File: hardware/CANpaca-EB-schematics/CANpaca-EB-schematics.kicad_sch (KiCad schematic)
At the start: 132 parts, among them J11 Conn_01x03_Male, J12 A2501WV-4P, J13 A2501WV-3P, J14 A2501WV-5P, J16 A2501WV-3P, J17 A2501WV-2P, J2 FAN_0, J4 Conn_01x03_Male, J5 FAN_1, J6 Screw_Terminal_01x02, J7 Conn_02x02_Odd_Even, J8 A2501WV-4P, J9 USB4110-GF-A_REVB, Q1 ES34000, Q2 ES34000, Q3 PSMN5R2-60YL, SW1 SW_DIP_x08, U1 SN65HVD1050D, U10 RP2040, U11 ADXL343, U2 SN74LVC1G14DRL, U3 TMC2130-LA, U4 LN5016, U5 AMS1117-3.3, U6 W25Q16, U7 USBLC6-2SC6, U8 MAX31865xTP, U9 SN74LVC1G32DVBR, Y1 12MHZ

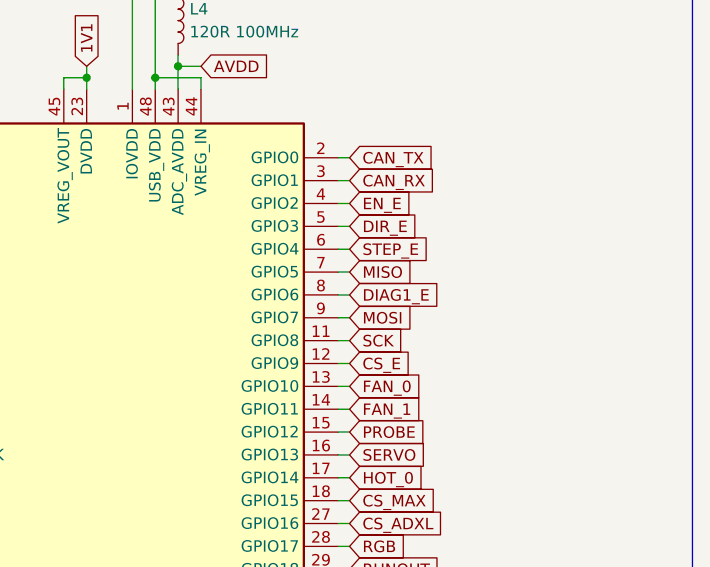
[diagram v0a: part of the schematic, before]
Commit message: added schematic pdf
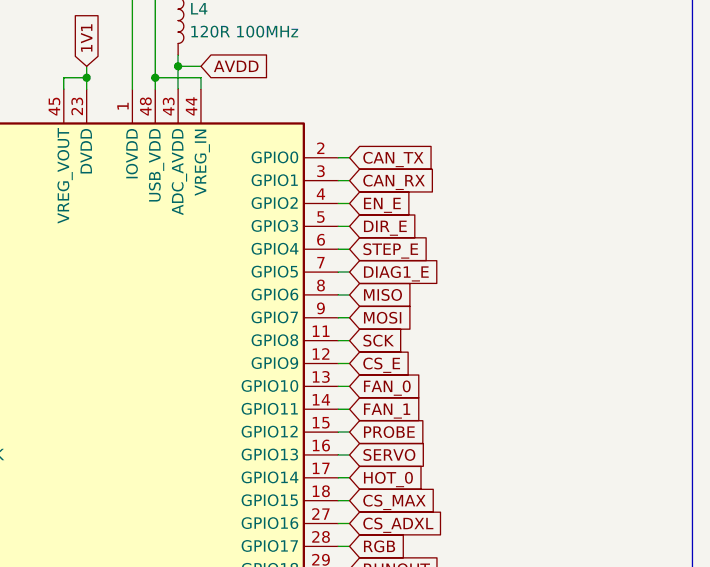
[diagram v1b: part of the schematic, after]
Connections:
- net DIAG1_E: now also U10.7 (GPIO5); no longer U10.8 (GPIO6)
- net MISO: now also U10.8 (GPIO6); no longer U10.7 (GPIO5)
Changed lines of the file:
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@@
+    (stroke (width 0) (type default) (color 0 0 0 0))
+  )
+  (wire (pts (xy 267.97 33.02) (xy 269.24 33.02))
+    (stroke (width 0) (type default) (color 0 0 0 0))
+  )
+  (wire (pts (xy 342.9 54.61) (xy 344.17 54.61))
+    (stroke (width 0) (type default) (color 0 0 0 0))
+  )
+  (wire (pts (xy 43.18 34.29) (xy 43.18 36.83))
+    (stroke (width 0) (type default) (color 0 0 0 0))
+  )
+  (wire (pts (xy 200.66 204.47) (xy 201.93 204.47))
+    (stroke (width 0) (type default) (color 0 0 0 0))
+  )
+  (wire (pts (xy 298.45 93.98) (xy 298.45 96.52))
+    (stroke (width 0) (type default) (color 0 0 0 0))
+  )
+  (wire (pts (xy 179.07 209.55) (xy 180.34 209.55))
+    (stroke (width 0) (type default) (color 0 0 0 0))
+  )
+  (wire (pts (xy 81.28 100.33) (xy 83.82 100.33))
+    (stroke (width 0) (type default) (color 0 0 0 0))
+  )
+  (wire (pts (xy 172.72 68.58) (xy 172.72 71.12))
+    (stroke (width 0) (type default) (color 0 0 0 0))
+  )
+  (wire (pts (xy 266.7 191.77) (xy 266.7 199.39))
+    (stroke (width 0) (type default) (color 0 0 0 0))
+  )
+  (wire (pts (xy 190.5 101.6) (xy 191.77 101.6))
+    (stroke (width 0) (type default) (color 0 0 0 0))
+  )
+  (wire (pts (xy 45.72 154.94) (xy 44.45 154.94))
+    (stroke (width 0) (type default) (color 0 0 0 0))
+  )
+  (wire (pts (xy 313.69 158.75) (xy 314.96 158.75))
+    (stroke (width 0) (type default) (color 0 0 0 0))
+  )
+  (wire (pts (xy 340.36 234.95) (xy 340.36 236.22))
+    (stroke (width 0) (type default) (color 0 0 0 0))
+  )
+  (wire (pts (xy 69.85 223.52) (xy 69.85 224.79))
+    (stroke (width 0) (type default) (color 0 0 0 0))
+  )
+  (polyline (pts (xy 114.3 132.08) (xy 15.24 132.08))
+    (stroke (width 0) (type default) (color 0 0 0 0))
+  )
+  (wire (pts (xy 279.4 93.98) (xy 278.13 93.98))
+    (stroke (width 0) (type default) (color 0 0 0 0))
+  )
+  (wire (pts (xy 83.82 97.79) (xy 83.82 93.98))
+    (stroke (width 0) (type default) (color 0 0 0 0))
+  )
+  (wire (pts (xy 186.69 167.64) (xy 186.69 172.72))
+    (stroke (width 0) (type default) (color 0 0 0 0))
+  )
+  (wire (pts (xy 162.56 71.12) (xy 163.83 71.12))
+    (stroke (width 0) (type default) (color 0 0 0 0))
+  )
+  (polyline (pts (xy 304.8 46.99) (xy 368.3 46.99))
+    (stroke (width 0) (type default) (color 0 0 0 0))
+  )
+  (wire (pts (xy 191.77 95.25) (xy 193.04 95.25))
+    (stroke (width 0) (type default) (color 0 0 0 0))
+  )
+  (wire (pts (xy 73.66 33.02) (xy 73.66 38.1))
+    (stroke (width 0) (type default) (color 0 0 0 0))
+  )
+  (wire (pts (xy 347.98 140.97) (xy 350.52 140.97))
+    (stroke (width 0) (type default) (color 0 0 0 0))
+  )
+  (wire (pts (xy 41.91 161.29) (xy 44.45 161.29))
+    (stroke (width 0) (type default) (color 0 0 0 0))
+  )
+  (wire (pts (xy 63.5 170.18) (xy 63.5 176.53))
+    (stroke (width 0) (type default) (color 0 0 0 0))
+  )
+  (wire (pts (xy 336.55 86.36) (xy 337.82 86.36))
+    (stroke (width 0) (type default) (color 0 0 0 0))
+  )
+  (wire (pts (xy 266.7 207.01) (xy 266.7 203.2))
+    (stroke (width 0) (type default) (color 0 0 0 0))
+  )
+  (wire (pts (xy 297.18 93.98) (xy 298.45 93.98))
+    (stroke (width 0) (type default) (color 0 0 0 0))
+  )
+  (wire (pts (xy 314.96 196.85) (xy 295.91 196.85))
+    (stroke (width 0) (type default) (color 0 0 0 0))
+  )
+  (wire (pts (xy 152.4 205.74) (xy 153.67 205.74))
+    (stroke (width 0) (type default) (color 0 0 0 0))
+  )
+  (wire (pts (xy 285.75 208.28) (xy 285.75 203.2))
     (stroke (width 0) (type default) (color 0 0 0 0))
   )
@@
     (stroke (width 0) (type default) (color 0 0 0 0))
   )
-  (wire (pts (xy 267.97 33.02) (xy 269.24 33.02))
-    (stroke (width 0) (type default) (color 0 0 0 0))
-  )
-  (wire (pts (xy 342.9 54.61) (xy 344.17 54.61))
-    (stroke (width 0) (type default) (color 0 0 0 0))
-  )
-  (wire (pts (xy 43.18 34.29) (xy 43.18 36.83))
-    (stroke (width 0) (type default) (color 0 0 0 0))
-  )
-  (wire (pts (xy 200.66 204.47) (xy 201.93 204.47))
-    (stroke (width 0) (type default) (color 0 0 0 0))
-  )
-  (wire (pts (xy 298.45 93.98) (xy 298.45 96.52))
-    (stroke (width 0) (type default) (color 0 0 0 0))
-  )
-  (wire (pts (xy 179.07 209.55) (xy 180.34 209.55))
-    (stroke (width 0) (type default) (color 0 0 0 0))
-  )
-  (wire (pts (xy 81.28 100.33) (xy 83.82 100.33))
-    (stroke (width 0) (type default) (color 0 0 0 0))
-  )
-  (wire (pts (xy 172.72 68.58) (xy 172.72 71.12))
-    (stroke (width 0) (type default) (color 0 0 0 0))
-  )
-  (wire (pts (xy 266.7 191.77) (xy 266.7 199.39))
-    (stroke (width 0) (type default) (color 0 0 0 0))
-  )
-  (wire (pts (xy 190.5 101.6) (xy 191.77 101.6))
-    (stroke (width 0) (type default) (color 0 0 0 0))
-  )
-  (wire (pts (xy 45.72 154.94) (xy 44.45 154.94))
-    (stroke (width 0) (type default) (color 0 0 0 0))
-  )
-  (wire (pts (xy 313.69 158.75) (xy 314.96 158.75))
-    (stroke (width 0) (type default) (color 0 0 0 0))
-  )
-  (wire (pts (xy 340.36 234.95) (xy 340.36 236.22))
-    (stroke (width 0) (type default) (color 0 0 0 0))
-  )
-  (wire (pts (xy 69.85 223.52) (xy 69.85 224.79))
-    (stroke (width 0) (type default) (color 0 0 0 0))
-  )
-  (polyline (pts (xy 114.3 132.08) (xy 15.24 132.08))
-    (stroke (width 0) (type default) (color 0 0 0 0))
-  )
-  (wire (pts (xy 279.4 93.98) (xy 278.13 93.98))
-    (stroke (width 0) (type default) (color 0 0 0 0))
-  )
-  (wire (pts (xy 83.82 97.79) (xy 83.82 93.98))
-    (stroke (width 0) (type default) (color 0 0 0 0))
-  )
-  (wire (pts (xy 186.69 167.64) (xy 186.69 172.72))
-    (stroke (width 0) (type default) (color 0 0 0 0))
-  )
-  (wire (pts (xy 162.56 71.12) (xy 163.83 71.12))
-    (stroke (width 0) (type default) (color 0 0 0 0))
-  )
-  (polyline (pts (xy 304.8 46.99) (xy 368.3 46.99))
-    (stroke (width 0) (type default) (color 0 0 0 0))
-  )
-  (wire (pts (xy 191.77 95.25) (xy 193.04 95.25))
-    (stroke (width 0) (type default) (color 0 0 0 0))
-  )
-  (wire (pts (xy 73.66 33.02) (xy 73.66 38.1))
-    (stroke (width 0) (type default) (color 0 0 0 0))
-  )
-  (wire (pts (xy 347.98 140.97) (xy 350.52 140.97))
-    (stroke (width 0) (type default) (color 0 0 0 0))
-  )
-  (wire (pts (xy 41.91 161.29) (xy 44.45 161.29))
-    (stroke (width 0) (type default) (color 0 0 0 0))
-  )
-  (wire (pts (xy 63.5 170.18) (xy 63.5 176.53))
-    (stroke (width 0) (type default) (color 0 0 0 0))
-  )
-  (wire (pts (xy 336.55 86.36) (xy 337.82 86.36))
-    (stroke (width 0) (type default) (color 0 0 0 0))
-  )
-  (wire (pts (xy 266.7 207.01) (xy 266.7 203.2))
-    (stroke (width 0) (type default) (color 0 0 0 0))
-  )
-  (wire (pts (xy 297.18 93.98) (xy 298.45 93.98))
-    (stroke (width 0) (type default) (color 0 0 0 0))
-  )
-  (wire (pts (xy 314.96 196.85) (xy 295.91 196.85))
-    (stroke (width 0) (type default) (color 0 0 0 0))
-  )
-  (wire (pts (xy 152.4 205.74) (xy 153.67 205.74))
-    (stroke (width 0) (type default) (color 0 0 0 0))
-  )
-  (wire (pts (xy 285.75 208.28) (xy 285.75 203.2))
-    (stroke (width 0) (type default) (color 0 0 0 0))
-  )
   (wire (pts (xy 314.96 86.36) (xy 314.96 92.71))
     (stroke (width 0) (type default) (color 0 0 0 0))
@@
     (stroke (width 0) (type default) (color 0 0 0 0))
   )
+  (wire (pts (xy 365.76 163.83) (xy 367.03 163.83))
+    (stroke (width 0) (type default) (color 0 0 0 0))
+  )
   (wire (pts (xy 190.5 156.21) (xy 190.5 172.72))
     (stroke (width 0) (type default) (color 0 0 0 0))
@@
   )
   (wire (pts (xy 80.01 147.32) (xy 81.28 147.32))
-    (stroke (width 0) (type default) (color 0 0 0 0))
-  )
-  (wire (pts (xy 365.76 163.83) (xy 367.03 163.83))
     (stroke (width 0) (type default) (color 0 0 0 0))
   )
@@
     )
   )
-  (global_label "MISO" (shape input) (at 367.03 163.83 0) (fields_autoplaced)
-    (effects (font (size 1.27 1.27)) (justify left))
-    (property "Intersheet References" "${INTERSHEET_REFS}" (id 0) (at 374.0393 163.7506 0)
+  (global_label "MISO" (shape input) (at 367.03 166.37 0) (fields_autoplaced)
+    (effects (font (size 1.27 1.27)) (justify left))
+    (property "Intersheet References" "${INTERSHEET_REFS}" (id 0) (at 374.0393 166.2906 0)
       (effects (font (size 1.27 1.27)) (justify left) hide)
     )
@@
     )
   )
-  (global_label "DIAG1_E" (shape input) (at 367.03 166.37 0) (fields_autoplaced)
-    (effects (font (size 1.27 1.27)) (justify left))
-    (property "Intersheet References" "${INTERSHEET_REFS}" (id 0) (at 377.0026 166.2906 0)
-      (effects (font (size 1.27 1.27)) (justify left) hide)
-    )
+  (global_label "DIAG1_E" (shape input) (at 367.03 163.83 0) (fields_autoplaced)
+    (effects (font (size 1.27 1.27)) (justify left))
+    (property "Intersheet References" "${INTERSHEET_REFS}" (id 0) (at 377.0026 163.7506 0)
+      (effects (font (size 1.27 1.27)) (justify left) hide)
+    )
